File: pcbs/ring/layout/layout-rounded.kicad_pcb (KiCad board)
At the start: 2 copper layers, 59.8 x 6.2 mm, 61 parts, among them J1 ?, Q1 CSD13380F3T, Q2 CSD13380F3T, U1 BQ27427YZFR, U2 BQ29700, U3 nRF52833-QDAA, U4 MAX30102EFD+T, U5 LSM6DSOX, U6 TMP117AIDRVR, U7 TPS7A2018PDQN, Y1 32MHz, Y2 32.768kHz

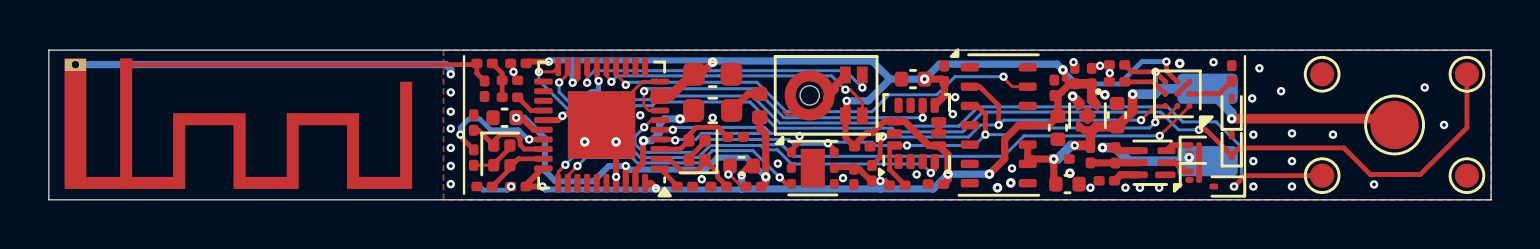
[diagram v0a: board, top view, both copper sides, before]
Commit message: rounded
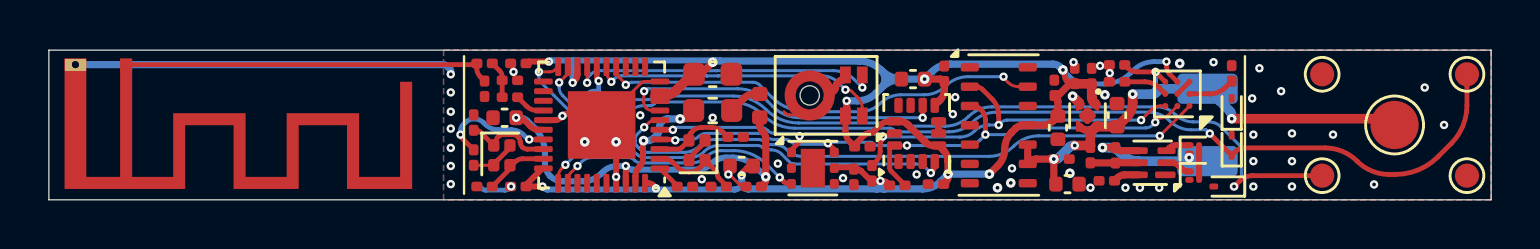
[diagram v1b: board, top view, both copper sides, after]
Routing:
- net swdclk: track 46.0 -> 44.9 mm
- net swdio: track 37.4 -> 36.7 mm
- net cpu.dec4_6: track 18.2 -> 17.7 mm

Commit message: more vias
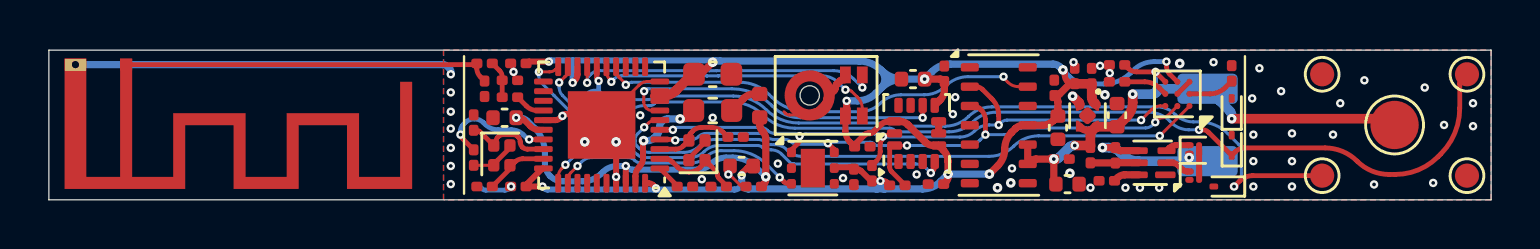
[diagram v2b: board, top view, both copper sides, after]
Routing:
- net GND: vias 50 -> 55
